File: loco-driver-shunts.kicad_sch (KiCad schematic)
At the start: 0 parts

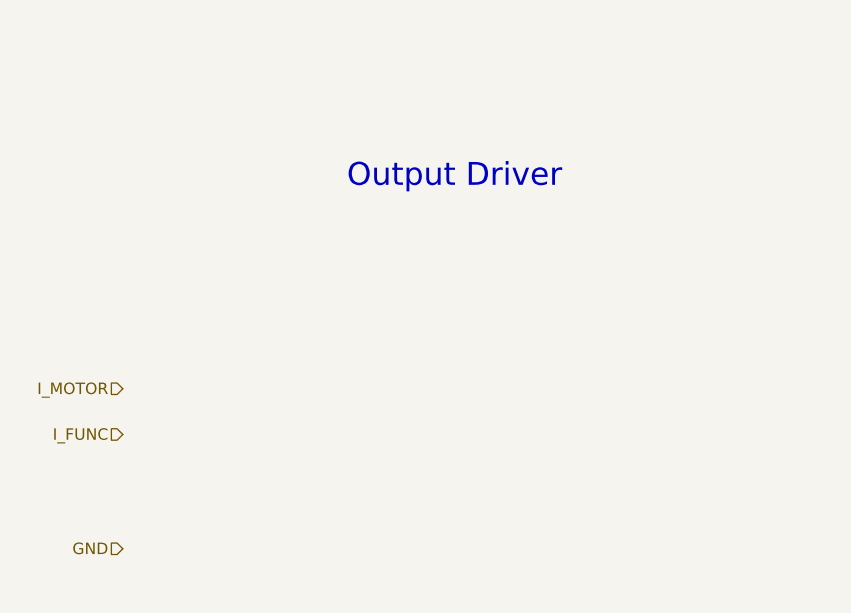
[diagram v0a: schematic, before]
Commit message: Fix - ERC updates
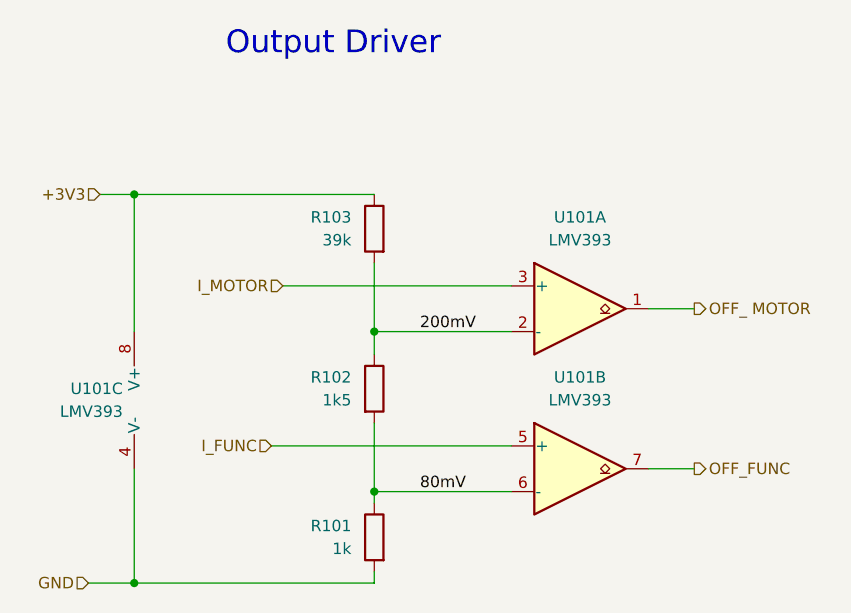
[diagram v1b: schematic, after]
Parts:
- added R101: 1k, symbol Device:R
- added R102: 1k5, symbol Device:R
- added R103: 39k, symbol Device:R
- added U101: LMV393, symbol Comparator:LMV393
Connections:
- net GND: now also R101.2, U101.4 (V-)
- net I_FUNC: now also U101.5 (+)
- net I_MOTOR: now also U101.3 (+)
- new net +3V3: R103.1, U101.8 (V+)
- new net 200mV: R102.1, R103.2, U101.2 (-)
- new net 80mV: R101.1, R102.2, U101.6 (-)
- new net OFF_ MOTOR: U101.1
- new net OFF_FUNC: U101.7
